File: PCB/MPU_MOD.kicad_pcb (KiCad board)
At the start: 6 copper layers, 50 x 50 mm, 295 parts, among them J501 MEM2090-00-145-00-A_REVA, J701 FTSH-107-01-L-DV-K-A, J801 USB4215-03-A_REVA, J901 73412-0110, U201 STC3115IQT, U202 BQ25606RGER, U203 STPMIC1APQR, U301 STM32MP157FABx, U401 MT41K256M16TW-107_P, U501 EMMC04G-W627-M06U, U502 HSP051-4M10, U503 HSP051-4M10, U701 HSP051-4M10, U702 HSP051-4M10, U801 FUSB302BMPX, U802 HSP051-4M10, U901 LBEE5PK2AE-771, Y601 NX2012SA-32.768K, Y701 ECS-2520MVQ-240

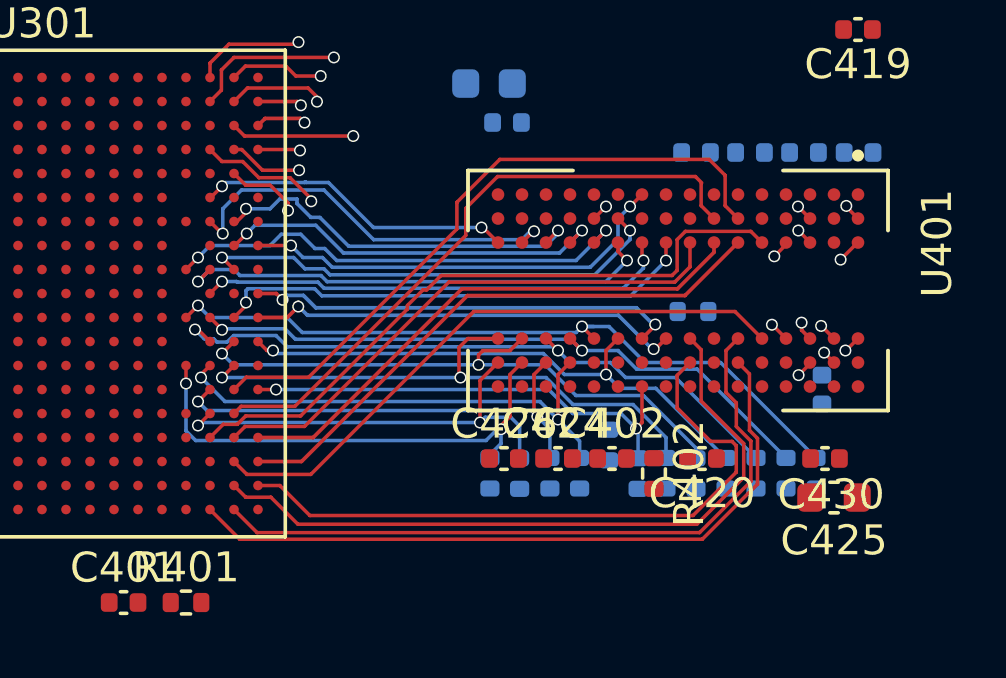
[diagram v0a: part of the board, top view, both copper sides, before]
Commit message: PCB_UPDATE
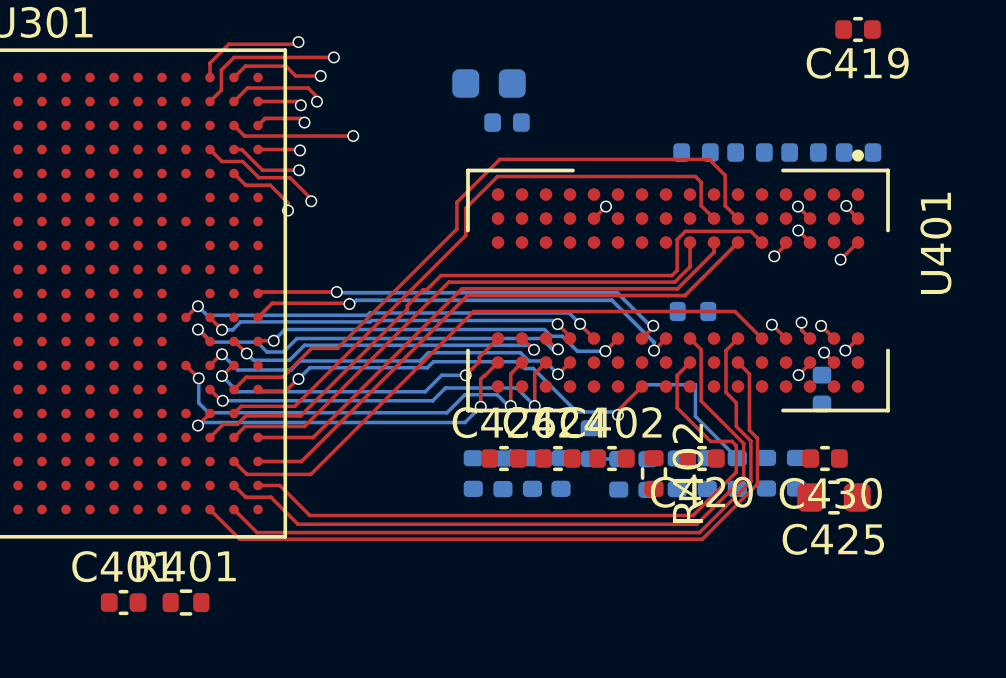
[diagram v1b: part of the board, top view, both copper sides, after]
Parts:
- moved R420 3.50 mm to (97.3, 75.0)
- moved R422 2.28 mm to (100.2, 75.0)
- moved R407 1.63 mm to (102.2, 75.0)
- moved R414 1.55 mm to (94.4, 75.0)
- moved R418 0.65 mm to (104.2, 75.0)
- moved R430 0.65 mm to (105.2, 75.0)
- moved R426 0.65 mm to (99.2, 75.0)
- moved R417 0.63 mm to (101.2, 75.0)
- moved R404 0.62 mm to (98.3, 74.0)
- moved R410 0.58 mm to (96.3, 75.0)
- moved R412 0.44 mm to (95.4, 75.0)
- moved R416 0.38 mm to (103.2, 75.0)
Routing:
- net /DDR/DDR_RASN: track 16.3 -> 0.00 mm, vias 2 -> 0
- net /DDR/DDR_WEN: track 16.2 -> 0.00 mm, vias 2 -> 0
- net /DDR/DDR_CASN: track 15.9 -> 0.00 mm, vias 2 -> 0
- net /DDR/DDR_BA2: track 15.8 -> 0.00 mm, vias 2 -> 0
- net /DDR/DDR_CSN: track 15.8 -> 0.00 mm, vias 2 -> 0
- net /DDR/DDR_ODT: track 14.5 -> 0.00 mm, vias 2 -> 0
- net /DDR/DDR_A9: track 13.4 -> 0.00 mm, vias 2 -> 0
- net /DDR/DDR_A0: track 13.1 -> 0.00 mm, vias 2 -> 0
- net /DDR/DDR_A2: track 12.8 -> 0.00 mm, vias 2 -> 0
- net /DDR/DDR_A13: track 10.7 -> 0.00 mm, vias 2 -> 0
- net /DDR/DDR_A15: track 24.4 -> 14.3 mm
- net /DDR/DDR_A12: track 21.7 -> 12.6 mm
- net /DDR/DDR_A11: track 20.0 -> 11.1 mm
- net /DDR/DDR_A14: track 19.3 -> 10.8 mm
- net /DDR/DDR_A1: track 21.9 -> 13.8 mm
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
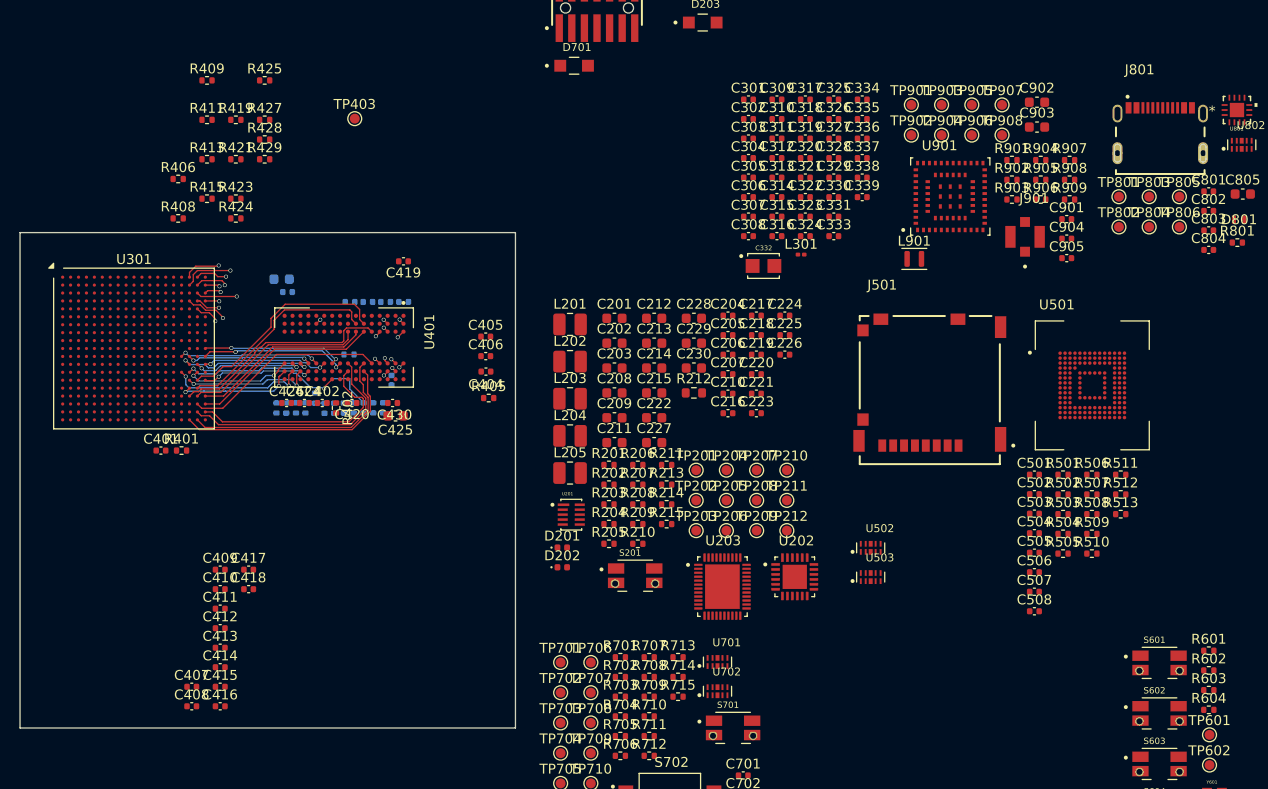
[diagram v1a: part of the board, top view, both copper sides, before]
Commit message: PCB_UPDATE
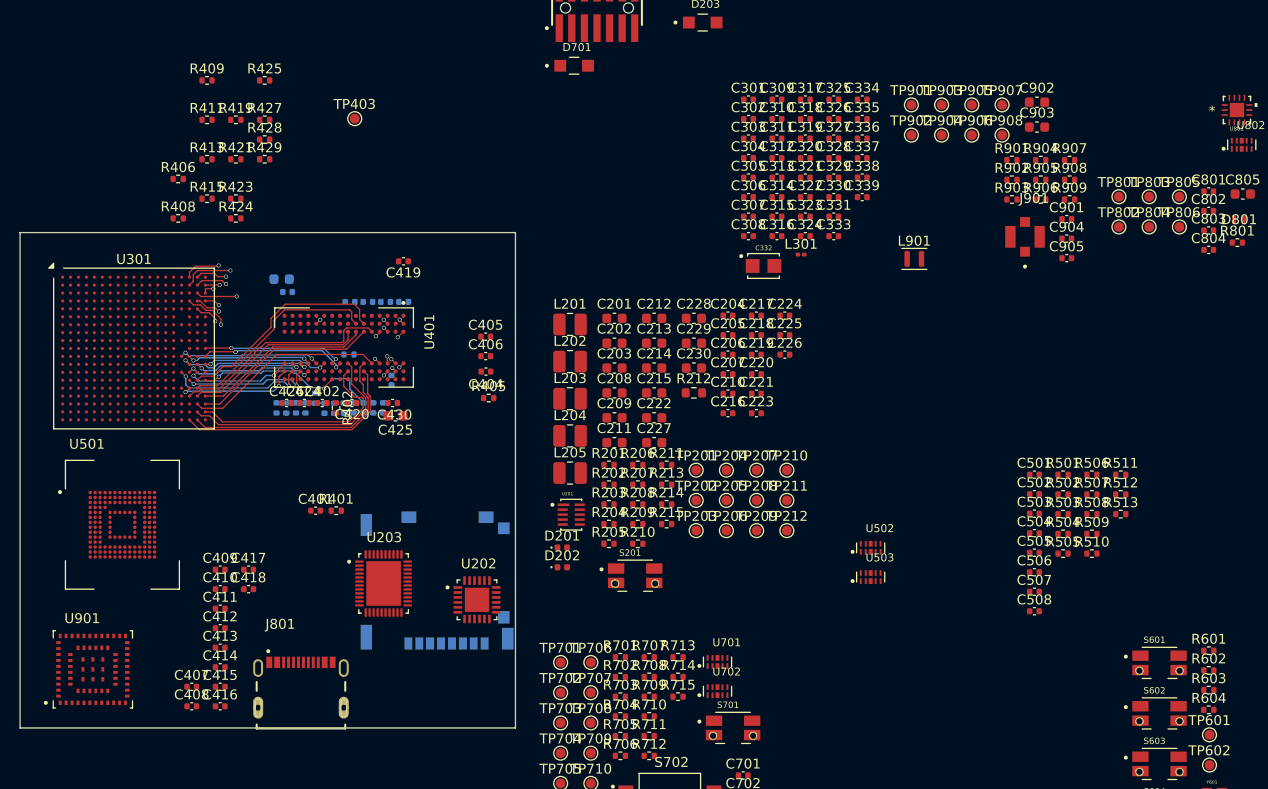
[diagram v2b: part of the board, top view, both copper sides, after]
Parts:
- J501: moved to B.Cu
- moved J801 103.2 mm to (96.8, 105.3)
- moved U501 98.9 mm to (78.8, 86.8)
- moved U901 98.8 mm to (75.8, 101.4)
- moved J501 53.6 mm to (110.6, 100.6), turned to 180 degrees
- moved U203 34.2 mm to (105.2, 92.7)
- moved U202 32.2 mm to (114.6, 94.4)
- moved C401 16.7 mm to (98.3, 85.4)
- moved R401 16.7 mm to (100.4, 85.4)
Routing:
- net /DDR/DDR_DQS0_P: track 21.7 -> 26.0 mm
- net /DDR/DDR_DQS0_N: track 22.5 -> 26.6 mm
- net /DDR/DDR_DQ6: track 20.2 -> 23.9 mm
- net /DDR/DDR_DQ4: track 23.1 -> 24.3 mm
- net /DDR/DDR_DQ2: track 23.8 -> 24.4 mm

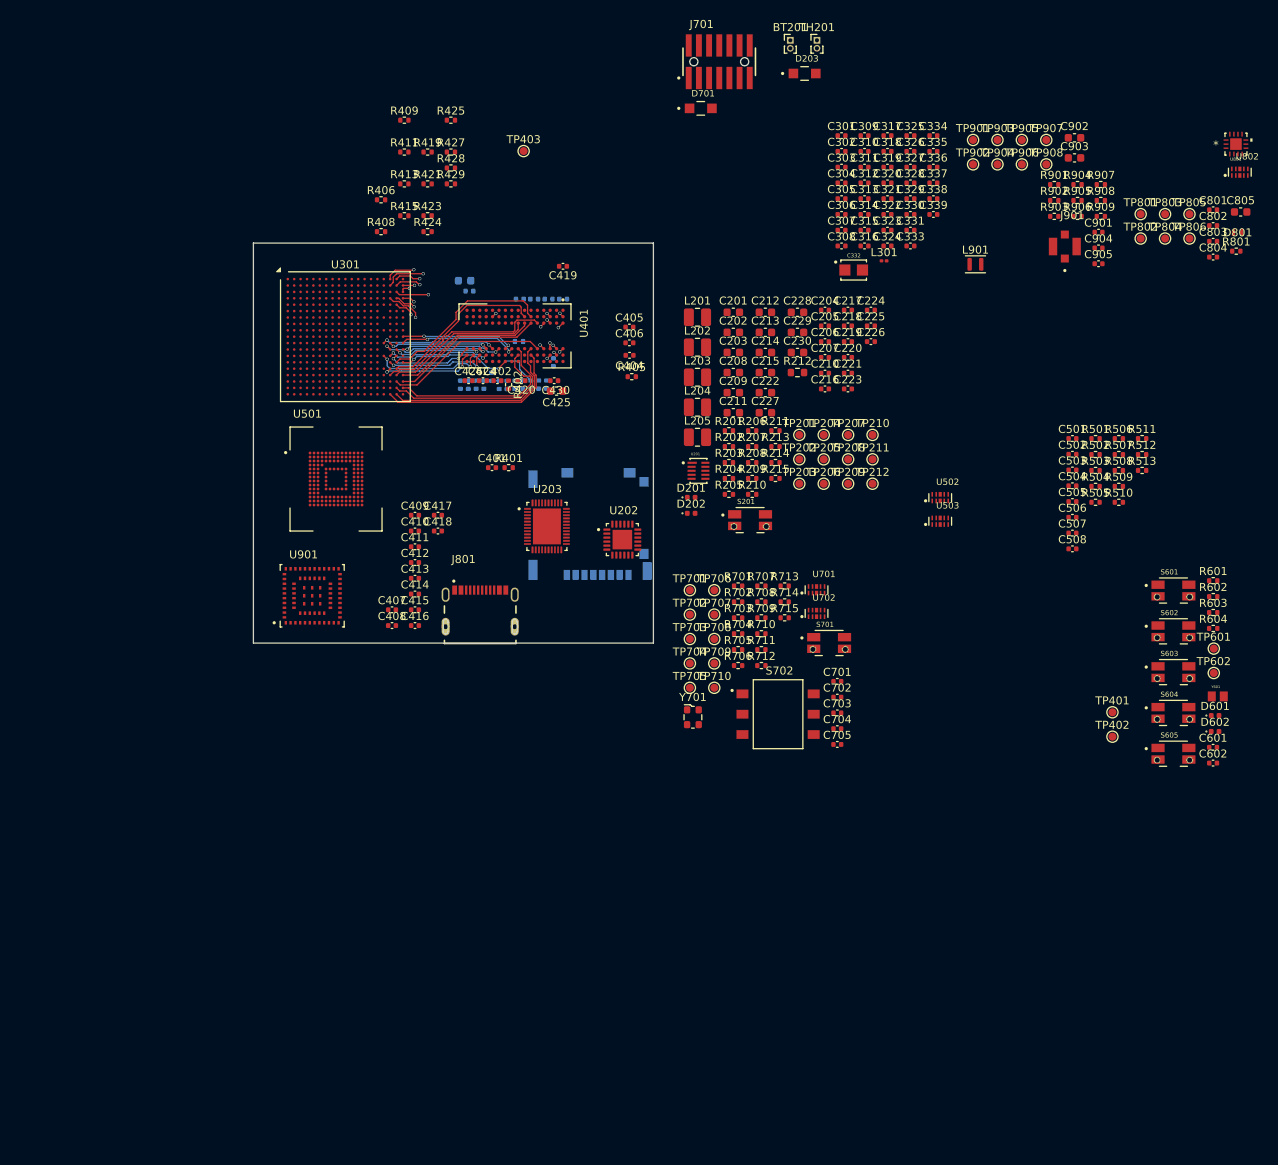
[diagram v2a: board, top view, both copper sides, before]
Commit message: PCB_UPDATE
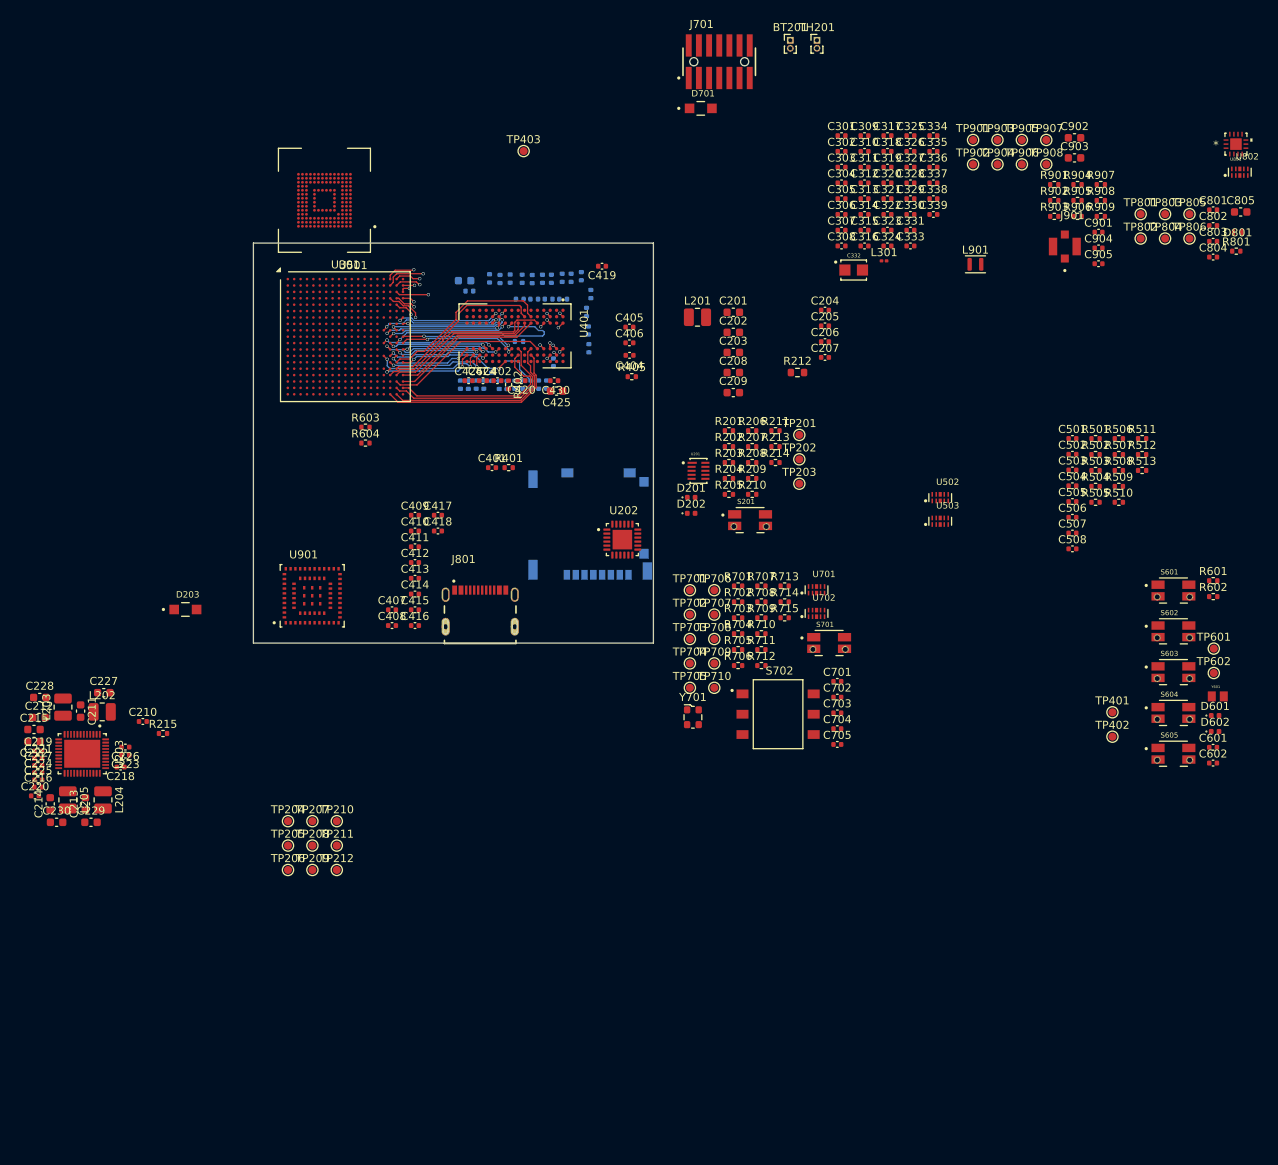
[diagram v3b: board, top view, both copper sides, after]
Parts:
- R406, R408, R409, R411, R413, R415, R419, R421, R423, R424, R425, R427, R428, R429: moved to B.Cu
- moved C224 119.1 mm to (41.6, 123.5)
- moved C225 118.6 mm to (41.6, 124.4)
- moved C217 116.1 mm to (41.6, 122.6)
- moved C220 115.5 mm to (41.2, 126.4)
- moved C219 113.4 mm to (41.6, 120.8)
- moved C221 112.1 mm to (41.6, 121.7)
- moved C216 110.2 mm to (41.6, 125.3)
- moved C230 109.7 mm to (43.9, 129.7)
- moved R603 108.5 mm to (82.5, 80.3)
- moved R604 108.5 mm to (82.5, 82.3)
- moved C229 107.5 mm to (48.2, 129.7)
- moved C218 106.3 mm to (51.9, 122.8), turned to 180 degrees
- moved C228 106.2 mm to (41.8, 114.1)
- moved C226 106.1 mm to (52.5, 120.3), turned to 180 degrees
- moved C214 105.7 mm to (43.1, 127.4), turned to 90 degrees
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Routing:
- net /DDR/DDR_RASN: track 0.00 -> 24.9 mm, vias 0 -> 2
- net /DDR/DDR_BA2: track 0.00 -> 15.6 mm, vias 0 -> 2
- net /DDR/DDR_CSN: track 0.00 -> 15.3 mm, vias 0 -> 2
- net /DDR/DDR_WEN: track 0.00 -> 15.3 mm, vias 0 -> 2
- net /DDR/DDR_CASN: track 0.00 -> 15.1 mm, vias 0 -> 2
- net /DDR/DDR_ODT: track 0.00 -> 14.1 mm, vias 0 -> 2
- net /DDR/DDR_BA0: track 0.57 -> 13.7 mm, vias 1 -> 2

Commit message: PCB_UPDATE
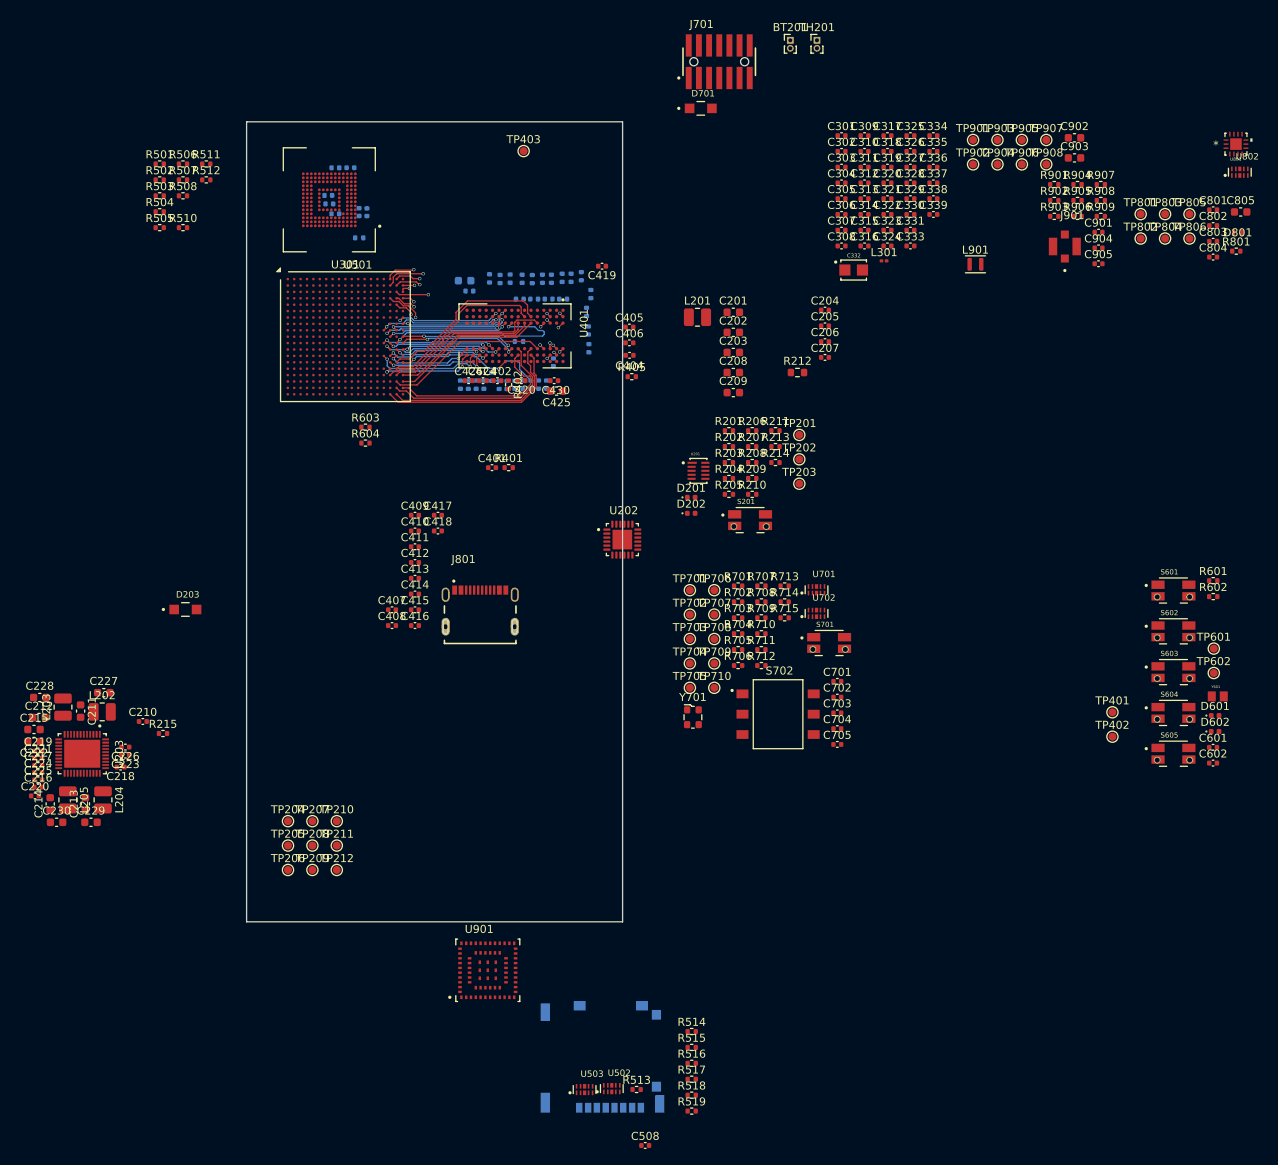
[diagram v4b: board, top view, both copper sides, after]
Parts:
- added R514: 47k, Resistor_SMD:R_0402_1005Metric, F.Cu at (123.3, 155.8)
- added R515: 47k, Resistor_SMD:R_0402_1005Metric, F.Cu at (123.3, 157.8)
- added R516: 47k, Resistor_SMD:R_0402_1005Metric, F.Cu at (123.3, 159.8)
- added R517: 47k, Resistor_SMD:R_0402_1005Metric, F.Cu at (123.3, 161.8)
- added R518: 47k, Resistor_SMD:R_0402_1005Metric, F.Cu at (123.3, 163.8)
- added R519: 47k, Resistor_SMD:R_0402_1005Metric, F.Cu at (123.3, 165.8)
- C501, C502, C503, C504, C505, C506, C507, R509: moved to B.Cu
- moved R501 121.9 mm to (56.8, 47.4)
- moved R502 121.9 mm to (56.8, 49.4)
- moved R503 121.9 mm to (56.8, 51.4)
- moved R504 121.9 mm to (56.8, 53.4)
- moved R505 121.9 mm to (56.8, 55.4)
- moved R506 121.9 mm to (59.7, 47.4)
- moved R507 121.9 mm to (59.7, 49.4)
- moved R508 121.9 mm to (59.7, 51.4)
- moved R510 121.9 mm to (59.7, 55.4)
- moved R511 121.9 mm to (62.6, 47.4)
- moved R512 121.9 mm to (62.6, 49.4)
- moved C507 101.1 mm to (80.6, 47.9)
- moved C505 100.6 mm to (77.9, 51.3)
- moved C504 100.3 mm to (78.8, 47.9)
- moved R509 99.9 mm to (81.7, 56.6), turned to 180 degrees
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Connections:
- net SYS_I2C_SCL renamed SYS_I2C4_SCL
- net SYS_I2C_SDA renamed SYS_I2C4_SDA
- TP905 pad 1: I2S3_SDO -> I2S1_SDO
- TP906 pad 1: I2S3_WS -> I2S1_WS
- TP907 pad 1: I2S3_CK -> I2S1_CK
- TP908 pad 1: I2S3_SDI -> I2S1_SDI
- U301 pad A2: unconnected-(U301D-PG15-PadA2) -> SDMMC3_CK
- U301 pad A3: unconnected-(U301C-PD0-PadA3) -> SDMMC3_CMD
- U301 pad A4: unconnected-(U301C-PD1-PadA4) -> SDMMC3_D0
- U301 pad B1: unconnected-(U301D-PE1-PadB1) -> UART8_TX_STM
- U301 pad B4: unconnected-(U301C-PD7-PadB4) -> SDMMC3_D3
- U301 pad C4: unconnected-(U301D-PE0-PadC4) -> UART8_RX_STM
- U301 pad D3: unconnected-(U301D-PE14-PadD3) -> UART8_RTS_STM
- U301 pad D6: unconnected-(U301C-PD4-PadD6) -> SDMMC3_D1
- U301 pad D7: unconnected-(U301C-PD5-PadD7) -> SDMMC3_D2
- U301 pad E1: unconnected-(U301D-PE15-PadE1) -> UART8_CTS_STM
- U301 pad P4: unconnected-(U301C-PA5-PadP4) -> I2S1_CK
- U301 pad R4: unconnected-(U301C-PA4-PadR4) -> I2S1_WS
- U301 pad T2: unconnected-(U301C-PC2-PadT2) -> I2S1_SDI
- U301 pad T5: unconnected-(U301C-PA6-PadT5) -> I2S1_SDI
- U301 pad T6: unconnected-(U301C-PA7-PadT6) -> I2S1_SDO
- U301 pad V2: unconnected-(U301C-PC1-PadV2) -> I2S1_SDO
- U301 pad V5: unconnected-(U301C-PB12-PadV5) -> I2S1_WS
- U301 pad W5: unconnected-(U301C-PB10-PadW5) -> I2S1_CK
- U901 pad 6: I2S3_SDI -> I2S1_SDI
- U901 pad 7: I2S3_CK -> I2S1_CK
- U901 pad 8: I2S3_WS -> I2S1_WS
- U901 pad 9: I2S3_SDO -> I2S1_SDO
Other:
- board size 50 x 50 mm -> 47 x 100 mm
